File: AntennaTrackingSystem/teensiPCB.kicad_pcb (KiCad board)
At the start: 2 copper layers, 45 x 84 mm, 13 parts, among them J1 screw terminal, J2 Conn_01x02, J5 UART1, J6 UART2, J7 I2C ext, SW1 SW_Push, U2 SAM-M10Q-00B

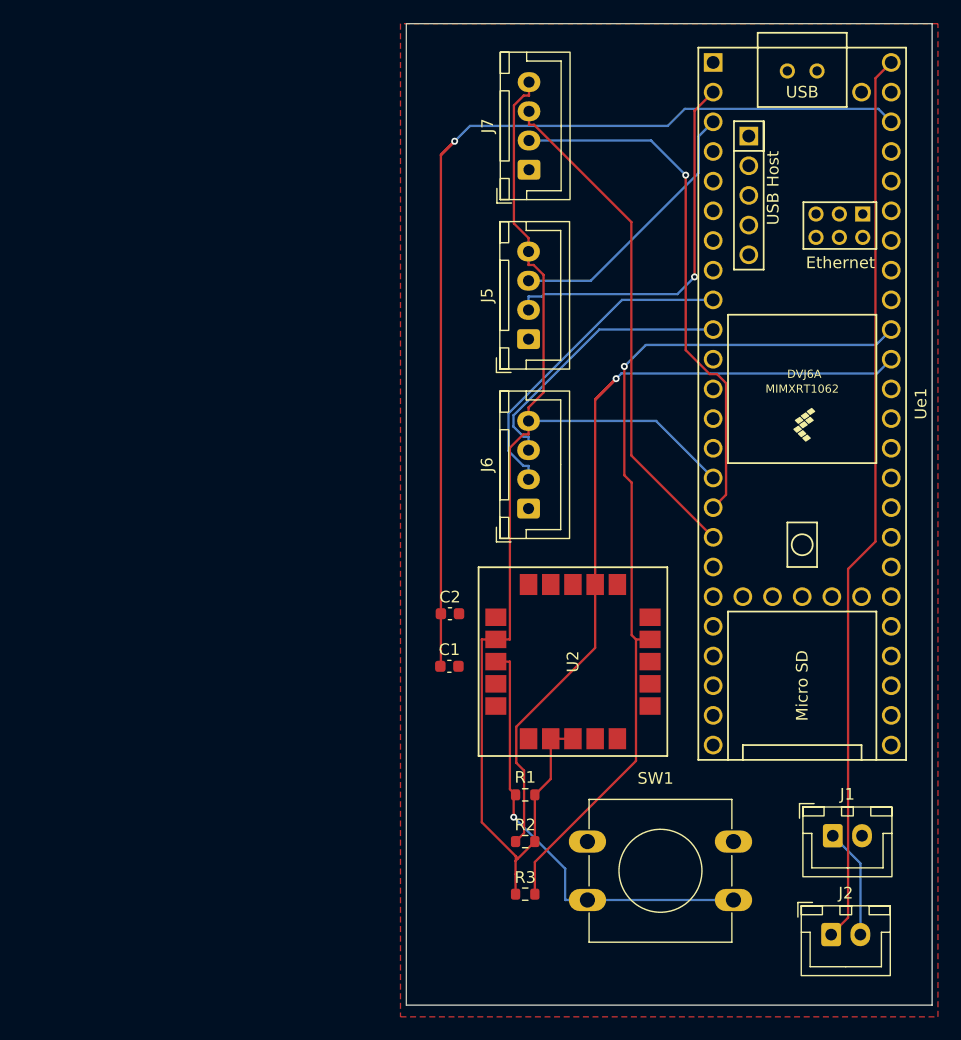
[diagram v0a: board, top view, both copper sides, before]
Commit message: teensy footprint
forgot to save
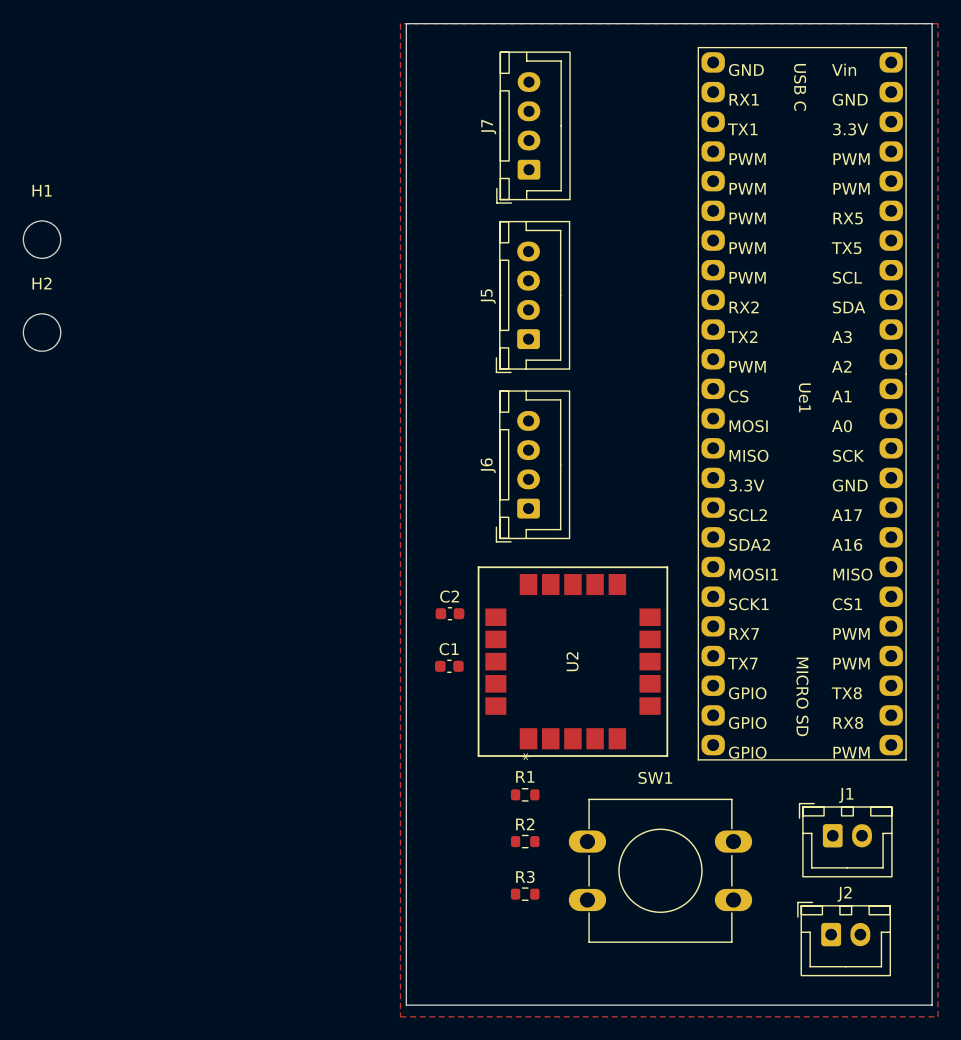
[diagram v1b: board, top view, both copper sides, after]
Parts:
- added H1: MountingHole, MountingHole:MountingHole_3.2mm_M3, F.Cu at (141.3, 77.5)
- added H2: MountingHole, MountingHole:MountingHole_3.2mm_M3, F.Cu at (141.3, 85.4)
- U2: footprint SAM M10Q footprint:SAM-M10Q_UBL -> SAM-M10Q:SAM-M10Q_UBL
- Ue1: footprint avionicsKiCadLibrary:Teensy41 -> teensy:teensy
- turned Ue1 to 0 degrees
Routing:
- net +3V3: track 108.3 -> 0.00 mm
- net Net-(C1-Pad1): track 91.1 -> 0.00 mm, vias 1 -> 0
- net Net-(U2-SCL): track 78.1 -> 0.00 mm, vias 1 -> 0
- net /+V: track 76.8 -> 0.00 mm
- net Net-(U2-SDA): track 74.5 -> 0.00 mm, vias 1 -> 0
- net Net-(J7-Pin_2): track 45.3 -> 0.00 mm, vias 1 -> 0
- net Net-(J7-Pin_3): track 43.2 -> 0.00 mm
- net Net-(U2-RESET_N): track 38.1 -> 0.00 mm, vias 1 -> 0
- net Net-(J5-Pin_2): track 32.5 -> 0.00 mm, vias 1 -> 0
- net Net-(J6-Pin_2): track 28.1 -> 0.00 mm
- net Net-(J6-Pin_3): track 23.9 -> 0.00 mm
- net Net-(J5-Pin_3): track 23.3 -> 0.00 mm
- net Net-(J1-Pin_1): track 9.44 -> 0.00 mm
